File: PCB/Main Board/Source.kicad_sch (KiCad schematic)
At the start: 50 parts, among them K1 AGQ200A12, Q1 2N7002, Q2 TIP41C, Q3 TIP42C, U2 DG201, U3 OPA2197xD, U4 OPA2197xD, U5 OPA2376xxD

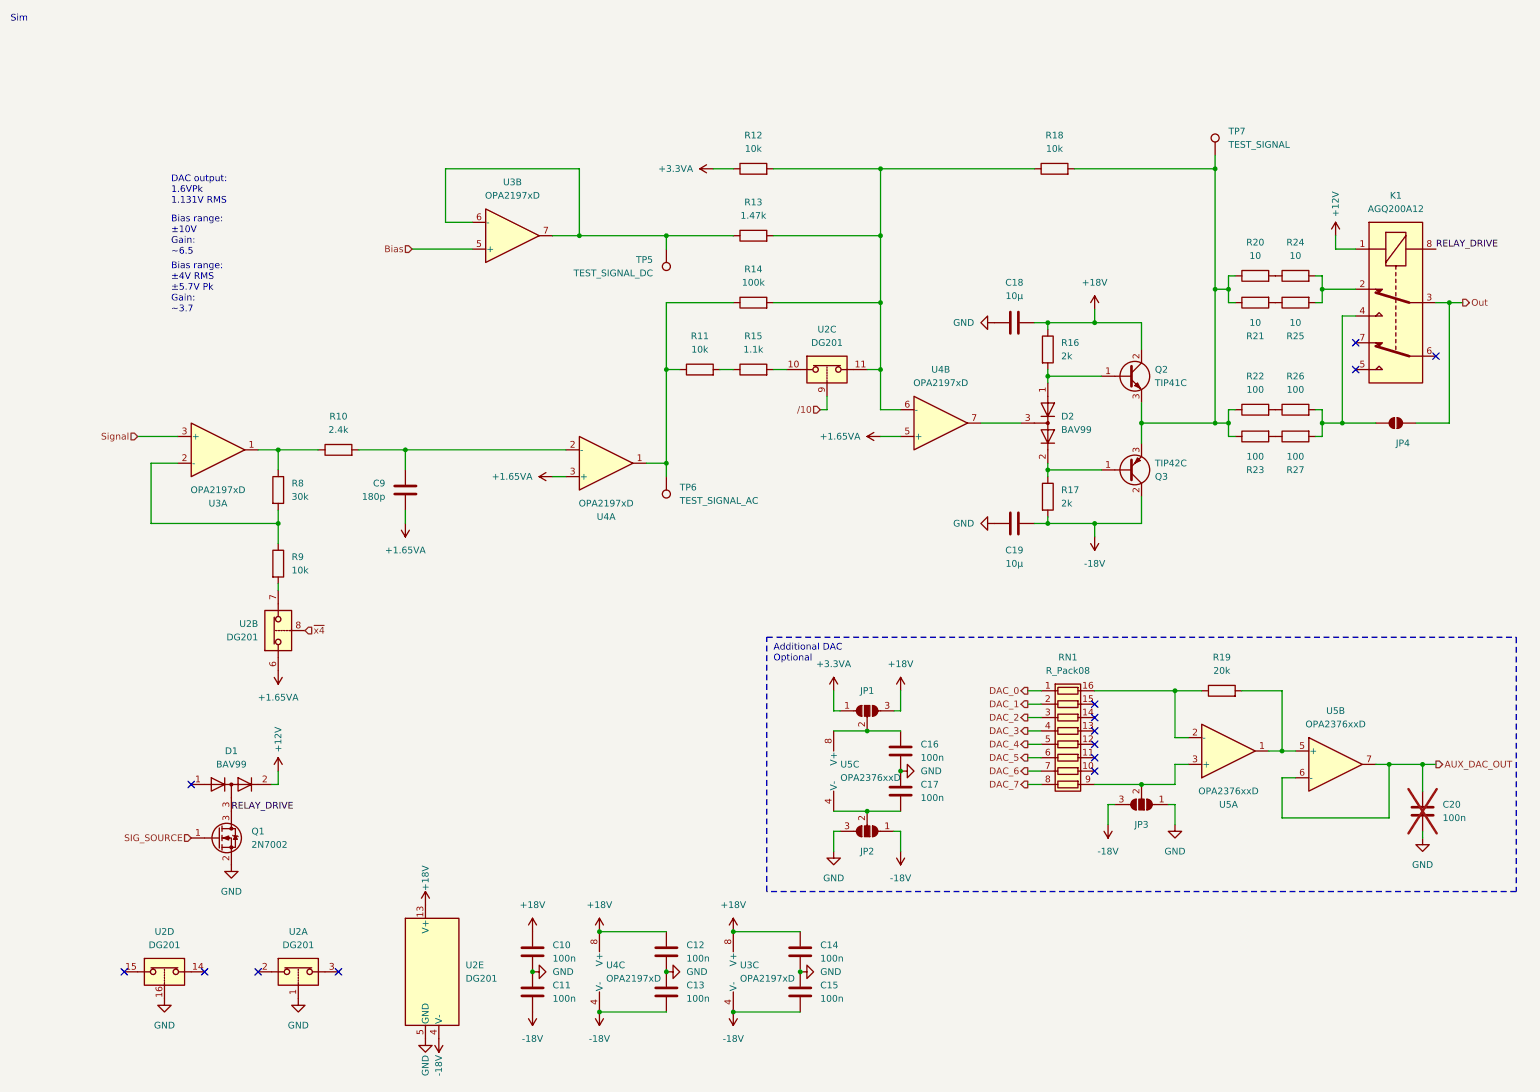
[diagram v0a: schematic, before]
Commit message: minor
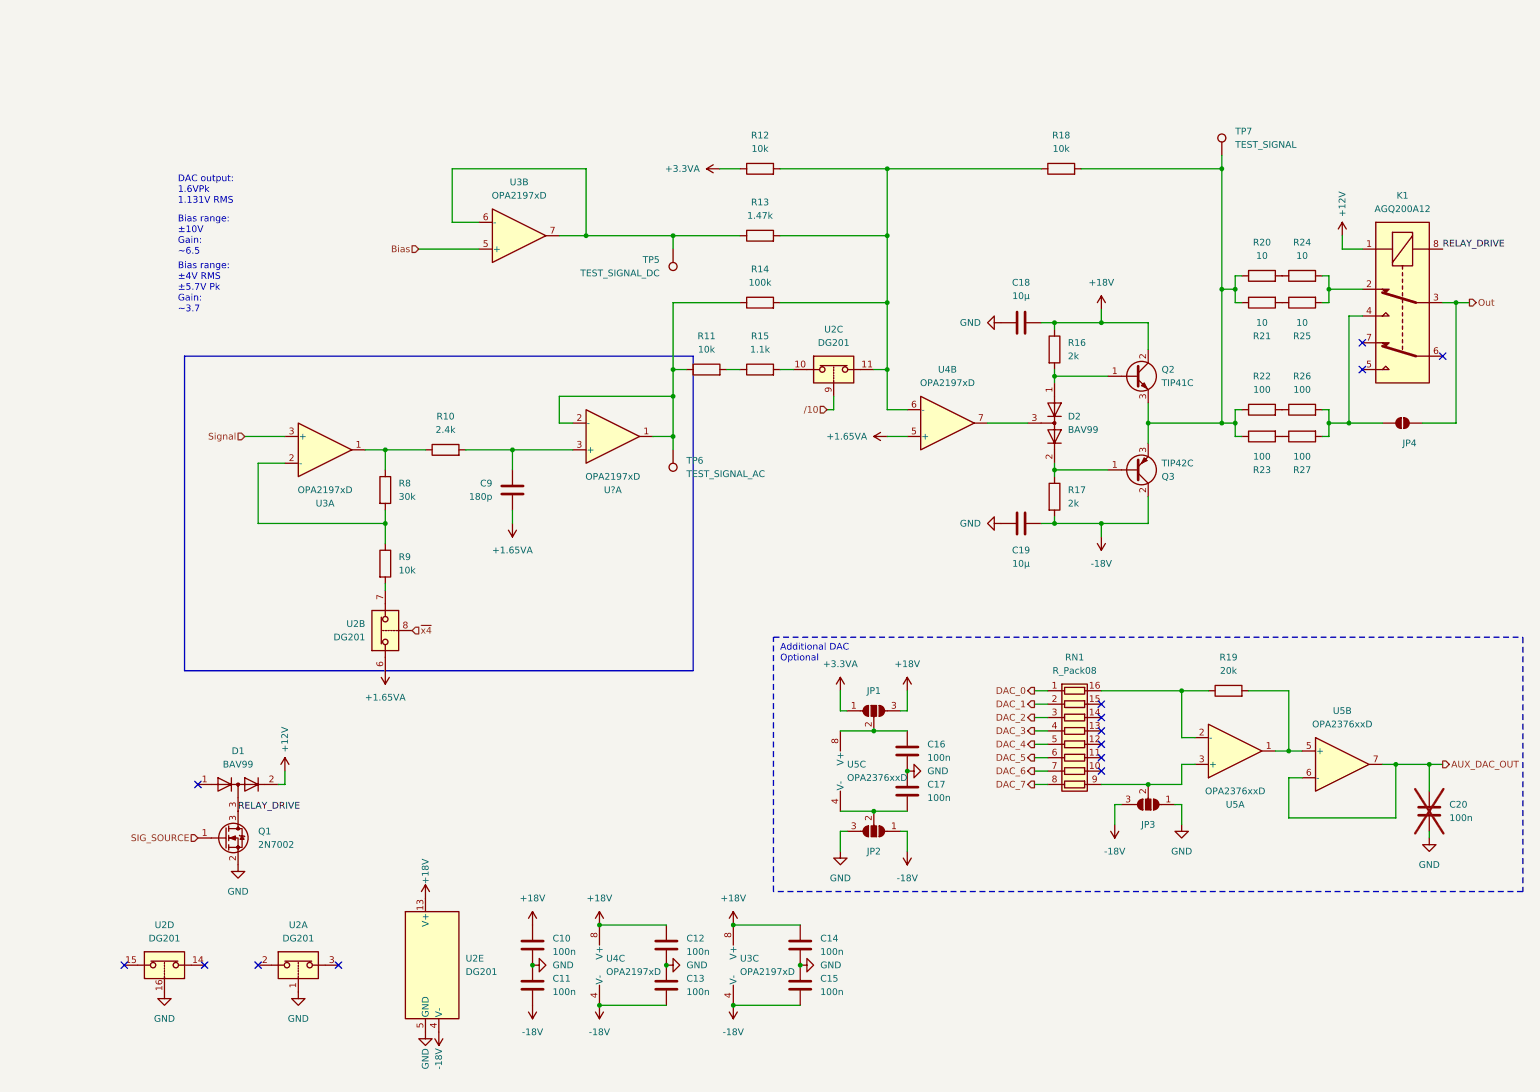
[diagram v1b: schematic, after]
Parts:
- removed unit 1 of U4
- added U?: OPA2197xD, Package_SO:SOIC-8_3.9x4.9mm_P1.27mm, symbol Amplifier_Operational:OPA2197xD
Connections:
- net at R11.1, R14.1, TP6.1: now also U?.1, U?.2 (-)
- net at C9.1, R10.2: now also U?.3 (+)
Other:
- note removed: "Sim"
- moved on the sheet: C10, C11, C12, C13, C14, C15, C16, C17, C18, C19, C20, C9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
